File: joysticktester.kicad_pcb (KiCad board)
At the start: 2 copper layers, 97 x 70 mm, 18 parts, among them J1 USB_OTG, J2 DB9_Male

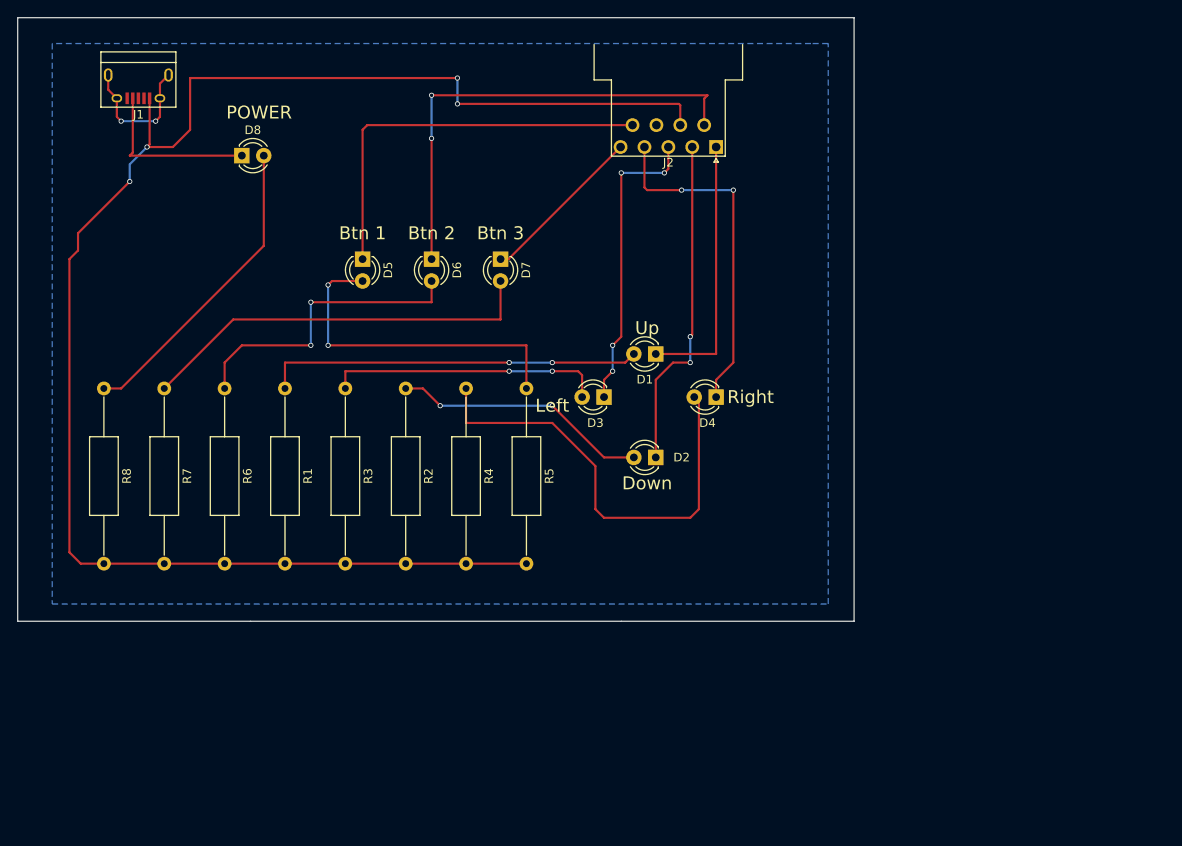
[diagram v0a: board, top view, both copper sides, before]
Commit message: new db9 connector
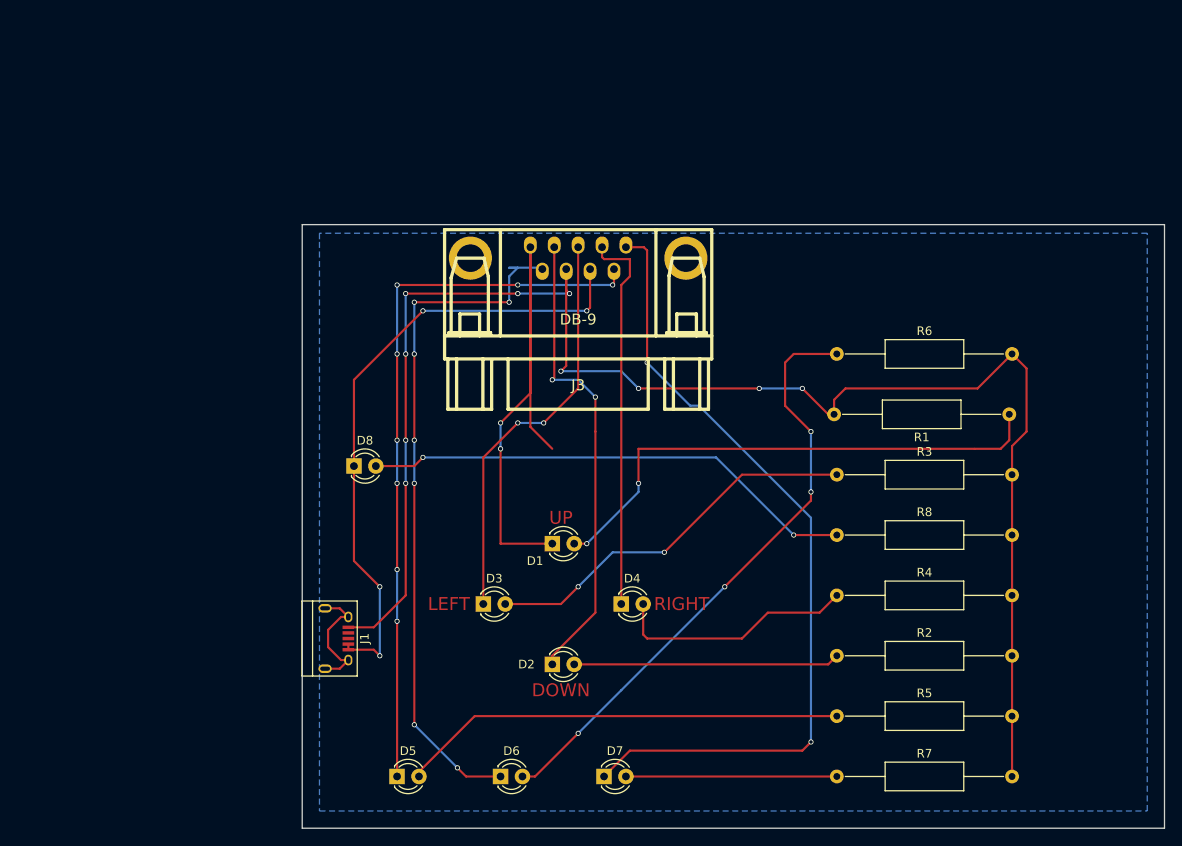
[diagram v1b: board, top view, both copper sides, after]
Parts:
- removed J2: DB9_Male, Connectors_DSub:DSUB-9_Male_Horizontal_Pitch2.77x2.54mm_EdgePinOffset9.40mm
- added J3: DB-9, w_conn_d-sub:DB_9M, F.Cu at (103.0, 61.0)
- moved R7 90.0 mm to (133.0, 114.0), turned to 0 degrees
- moved R8 86.7 mm to (133.0, 86.0), turned to 0 degrees
- moved R1 84.1 mm to (153.0, 72.0), turned to 180 degrees
- moved R6 71.1 mm to (133.0, 65.0), turned to 0 degrees
- moved J1 68.0 mm to (75.0, 98.0), turned to 270 degrees
- moved D7 61.2 mm to (106.0, 114.0), turned to 0 degrees
- moved D6 60.5 mm to (94.0, 114.0), turned to 0 degrees
- moved D5 60.1 mm to (82.0, 114.0), turned to 0 degrees
- moved R2 58.8 mm to (133.0, 100.0), turned to 0 degrees
- moved R3 57.9 mm to (133.0, 79.0), turned to 0 degrees
- moved R5 52.3 mm to (133.0, 107.0), turned to 0 degrees
- moved R4 49.2 mm to (133.0, 93.0), turned to 0 degrees
- moved D8 38.3 mm to (77.0, 78.0)
- moved D3 27.8 mm to (92.0, 94.0), turned to 0 degrees
- moved D2 26.8 mm to (100.0, 101.0), turned to 0 degrees
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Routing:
- net /BUTTON3: track 19.3 -> 93.7 mm, vias 0 -> 2
- net /GROUND: track 19.8 -> 73.1 mm, vias 0 -> 4
- net /BUTTON1: track 46.5 -> 83.9 mm, vias 0 -> 8
- net /UP: track 31.0 -> 66.2 mm, vias 0 -> 2
- net Net-(D6-Pad2): track 35.3 -> 70.4 mm, vias 2 -> 4
- net /BUTTON2: track 54.6 -> 81.8 mm, vias 2 -> 8
- net Net-(D4-Pad2): track 52.1 -> 28.3 mm
- net Net-(D7-Pad2): track 46.8 -> 24.5 mm
- net Net-(D8-Pad2): track 35.9 -> 57.6 mm, vias 0 -> 2
- net Net-(D1-Pad2): track 43.9 -> 61.4 mm
- net /DOWN: track 38.9 -> 54.4 mm
- net /LEFT: track 35.0 -> 47.7 mm, vias 4 -> 2
- net Net-(D5-Pad2): track 39.2 -> 51.7 mm, vias 2 -> 0
- net Net-(D3-Pad2): track 32.2 -> 44.7 mm
- net /RIGHT: track 40.0 -> 44.9 mm, vias 2 -> 0
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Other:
- board size 97 x 70 mm -> 100 x 70 mm
- board text added: "DOWN"
- board text added: "LEFT"
- board text added: "RIGHT"
- board text added: "UP"
- board text removed: "Btn 1"
- board text removed: "Btn 2"
- board text removed: "Btn 3"
- board text removed: "Down"
- board text removed: "Left"
- board text removed: "POWER"
- board text removed: "Right"
- board text removed: "Up"
- board text removed: "https://github.com/Ozzyboshi/AmigaJoystickTesterPCB"
